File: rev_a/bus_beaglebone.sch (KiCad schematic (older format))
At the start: 39 parts, among them J1 TERMINATE_JUMPER, J2 LED_JUMPER, Q1 FQP47P06, SW1 MJTP1243, U1 74HCT08, U2 MCP2562, U3 ATMEGA324_DIP40, X1 16MHz, X2 OSHW_LOGO

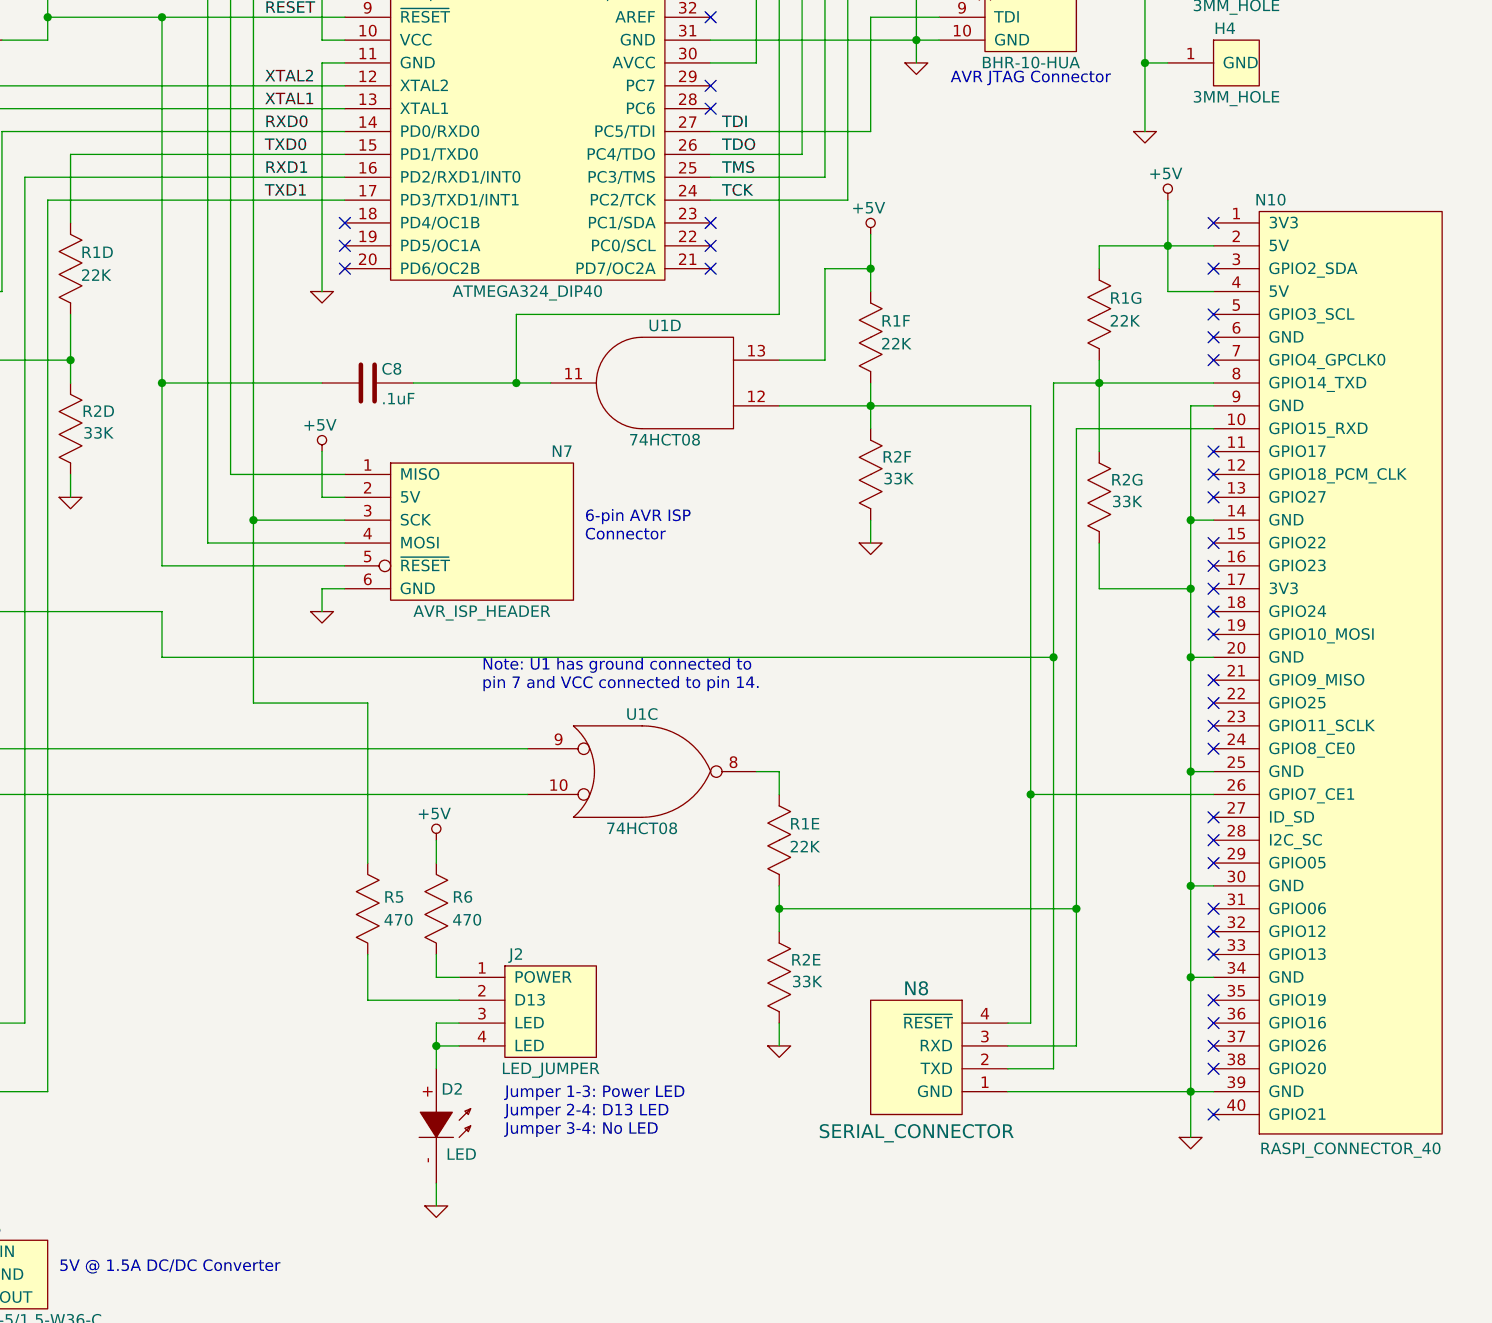
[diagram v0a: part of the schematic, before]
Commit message: Updated again.
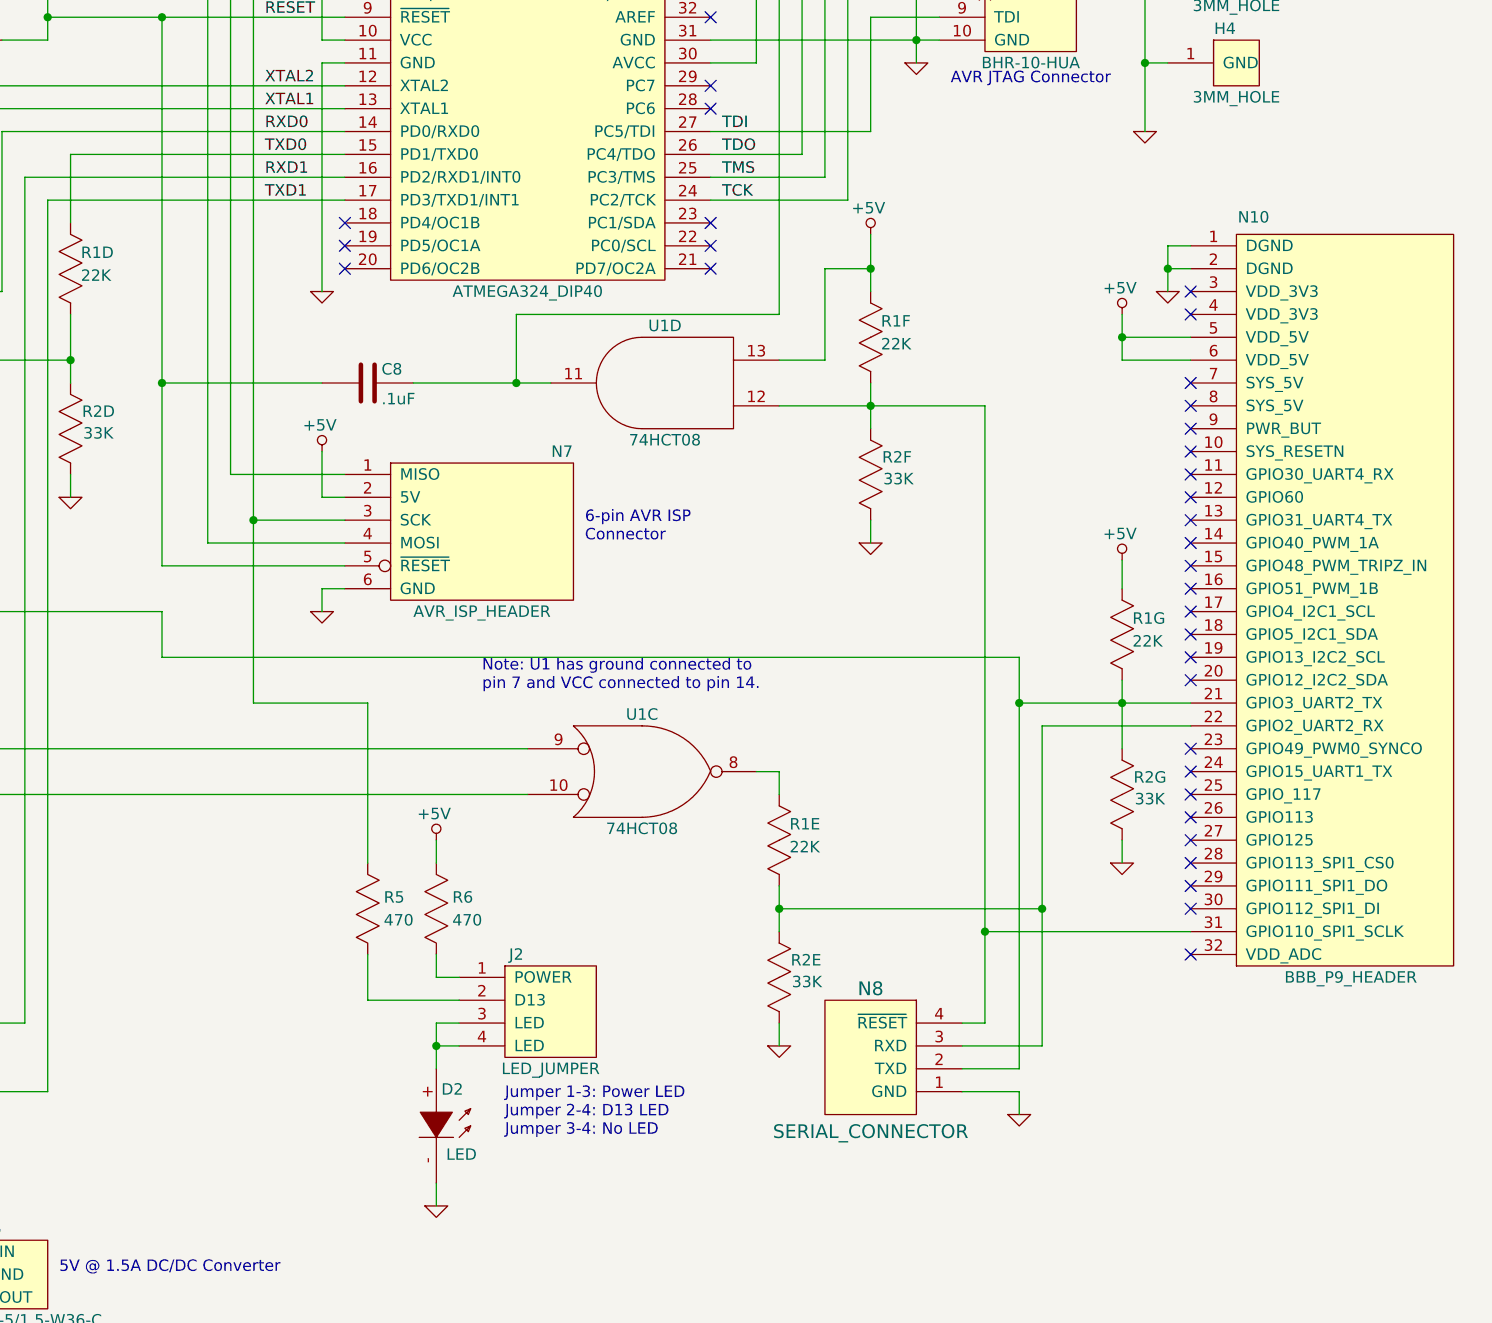
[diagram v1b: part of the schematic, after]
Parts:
- removed N10: RASPI_CONNECTOR_40, symbol RASPI_CONNECTOR_40
- added N10: BBB_P9_HEADER, symbol BBB_P9_HEADER
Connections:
- net +5V: now also N10.5 (VDD_5V), N10.6 (VDD_5V)
- net GND: now also N10.1 (DGND), N10.2 (DGND)
- net at N5.5 (RXD), N8.2 (TXD), R1.8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: now also N10.21 (GPIO3_UART2_TX)
- net at N8.3 (RXD), R1.6, R2.6: now also N10.22 (GPIO2_UART2_RX)
- net at N8.4 (~RESET), R1.7, R2.7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: now also N10.31 (GPIO110_SPI1_SCLK)
- no-connect marks 63 -> 60
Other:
- moved on the sheet: N8, R1G, R2G
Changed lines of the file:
@@
 L GND #PWR09
 U 1 1 53E41588
-P 9300 6600
-F 0 "#PWR09" H 9300 6600 30  0001 C CNN
-F 1 "GND" H 9300 6530 30  0001 C CNN
-F 2 "" H 9300 6600 60  0000 C CNN
-F 3 "" H 9300 6600 60  0000 C CNN
-	1    9300 6600
+P 8550 6500
+F 0 "#PWR09" H 8550 6500 30  0001 C CNN
+F 1 "GND" H 8550 6430 30  0001 C CNN
+F 2 "" H 8550 6500 60  0000 C CNN
+F 3 "" H 8550 6500 60  0000 C CNN
+	1    8550 6500
 	1    0    0    -1
 $EndComp
@@
 L +5V #PWR017
 U 1 1 53E51681
-P 9200 2500
-F 0 "#PWR017" H 9200 2590 20  0001 C CNN
-F 1 "+5V" H 9190 2615 50  0000 C CNN
-F 2 "" H 9200 2500 60  0000 C CNN
-F 3 "" H 9200 2500 60  0000 C CNN
-	1    9200 2500
+P 9000 3000
+F 0 "#PWR017" H 9000 3090 20  0001 C CNN
+F 1 "+5V" H 8990 3115 50  0000 C CNN
+F 2 "" H 9000 3000 60  0000 C CNN
+F 3 "" H 9000 3000 60  0000 C CNN
+	1    9000 3000
 	1    0    0    -1
 $EndComp
@@
 	1    0    0    -1
 $EndComp
-$Comp
-L RASPI_CONNECTOR_40 N10
-U 1 1 53E65B95
-P 10000 4450
-F 0 "N10" H 9650 6400 50  0000 C CNN
-F 1 "RASPI_CONNECTOR_40" H 10000 2250 50  0000 C CNN
-F 2 "" H 10000 5050 60  0000 C CNN
-F 3 "" H 10000 5050 60  0000 C CNN
-	1    10000 4450
-	1    0    0    -1
-$EndComp
-NoConn ~ 9400 2600
-NoConn ~ 9400 2800
-NoConn ~ 9400 3000
-NoConn ~ 9400 3100
-NoConn ~ 9400 3200
-NoConn ~ 9400 3600
-NoConn ~ 9400 3700
-NoConn ~ 9400 3800
-NoConn ~ 9400 4000
-NoConn ~ 9400 4100
-NoConn ~ 9400 4200
-NoConn ~ 9400 4300
-NoConn ~ 9400 4400
-NoConn ~ 9400 4600
-NoConn ~ 9400 4700
-NoConn ~ 9400 4800
-NoConn ~ 9400 4900
-NoConn ~ 9400 5200
-NoConn ~ 9400 5300
-NoConn ~ 9400 5400
-NoConn ~ 9400 5600
-NoConn ~ 9400 5700
-NoConn ~ 9400 5800
-NoConn ~ 9400 6000
-NoConn ~ 9400 6100
-NoConn ~ 9400 6200
-NoConn ~ 9400 6300
-NoConn ~ 9400 6500
 Text Notes 6650 4000 0    50   ~ 0
 6-pin AVR ISP\nConnector
@@
 L SERIAL_CONNECTOR N8
 U 1 1 53E7BE34
-P 8100 6250
-F 0 "N8" H 8100 6550 60  0000 C CNN
-F 1 "SERIAL_CONNECTOR" H 8100 5925 60  0000 C CNN
-F 2 "" H 8100 6250 60  0000 C CNN
-F 3 "" H 8100 6250 60  0000 C CNN
-	1    8100 6250
+P 7900 6250
+F 0 "N8" H 7900 6550 60  0000 C CNN
+F 1 "SERIAL_CONNECTOR" H 7900 5925 60  0000 C CNN
+F 2 "" H 7900 6250 60  0000 C CNN
+F 3 "" H 7900 6250 60  0000 C CNN
+	1    7900 6250
 	-1   0    0    -1
 $EndComp
@@
 	1300 3100 1900 3100
 Wire Wire Line
-	9300 3400 9300 6600
-Wire Wire Line
-	9300 3400 9400 3400
-Wire Wire Line
-	9400 5000 9300 5000
-Connection ~ 9300 5000
-Connection ~ 9300 5500
-Wire Wire Line
-	9400 3900 9300 3900
-Connection ~ 9300 3900
-Wire Wire Line
-	8800 3500 9400 3500
+	8650 4800 9300 4800
 Wire Wire Line
 	7500 5500 7500 5700
@@
 	3500 6900 3500 7300
 Wire Wire Line
-	9200 2900 9400 2900
-Wire Wire Line
-	9200 2500 9200 2900
-Wire Wire Line
-	8900 2700 9400 2700
-Connection ~ 9200 2700
+	9000 3200 9300 3200
+Wire Wire Line
+	9000 3000 9000 3200
 Wire Wire Line
 	2300 6400 2200 6400
@@
 	1600 5500 1600 5700
 Wire Wire Line
-	8700 3300 9400 3300
+	8550 4700 9300 4700
 Wire Wire Line
 	3500 1500 4300 1500
@@
 	1300 3200 4400 3200
 Wire Wire Line
-	8800 3500 8800 6200
-Wire Wire Line
-	8800 5600 7500 5600
+	8650 4800 8650 6200
+Wire Wire Line
+	8650 5600 7500 5600
 Connection ~ 7500 5600
 Wire Wire Line
@@
 	5200 1600 5600 1600
 Wire Wire Line
-	9400 5100 8600 5100
-Wire Wire Line
-	8600 3400 8600 6100
+	9300 5700 8400 5700
+Wire Wire Line
+	8400 3400 8400 6100
 Wire Wire Line
 	7500 1400 8200 1400
@@
 	6350 3000 7500 3000
 Wire Wire Line
-	7500 3400 8600 3400
+	7500 3400 8400 3400
 Wire Wire Line
 	5200 1600 5200 4700
@@
 	7900 3300 7900 3500
 Connection ~ 7900 3400
-Wire Wire Line
-	8900 2700 8900 2800
-Wire Wire Line
-	9400 4500 9300 4500
-Connection ~ 9300 4500
 Wire Wire Line
 	7500 3000 7500 1400
@@
 	7700 2400 7200 2400
 Wire Wire Line
-	8900 4200 9300 4200
-Connection ~ 9300 4200
-Wire Wire Line
-	8900 4200 8900 4000
-Wire Wire Line
-	8500 6400 9400 6400
-Connection ~ 9300 6400
-Wire Wire Line
-	9400 5500 9300 5500
-Wire Wire Line
-	9400 5900 9300 5900
-Connection ~ 9300 5900
-Wire Wire Line
-	4800 4500 8700 4500
-Wire Wire Line
-	8700 3300 8700 6300
-Wire Wire Line
-	8900 3200 8900 3600
-Connection ~ 8900 3300
+	9000 5400 9000 5300
+Wire Wire Line
+	4800 4500 8550 4500
+Wire Wire Line
+	8550 4500 8550 6300
+Wire Wire Line
+	9000 4600 9000 4900
+Connection ~ 9000 4700
 Wire Wire Line
 	4800 4100 5600 4100
@@
 	5500 3300 4800 3300
 Wire Wire Line
-	8600 6100 8500 6100
-Connection ~ 8600 5100
-Wire Wire Line
-	8700 6300 8500 6300
-Connection ~ 8700 4500
-Wire Wire Line
-	8800 6200 8500 6200
-Connection ~ 8800 5600
+	8400 6100 8300 6100
+Connection ~ 8400 5700
+Wire Wire Line
+	8550 6300 8300 6300
+Wire Wire Line
+	8650 6200 8300 6200
+Connection ~ 8650 5600
 Text Label 1150 7100 0    50   ~ 0
 BAT+
@@
 L R_VERT_SIP8 R1
 U 7 1 53E80F50
-P 8900 3000
-F 0 "R1" H 8945 3070 50  0000 L CNN
-F 1 "22K" H 8945 2970 50  0000 L CNN
-F 2 "" H 8900 3000 50  0000 C CNN
-F 3 "" H 8900 3000 50  0000 C CNN
-	7    8900 3000
+P 9000 4400
+F 0 "R1" H 9045 4470 50  0000 L CNN
+F 1 "22K" H 9045 4370 50  0000 L CNN
+F 2 "" H 9000 4400 50  0000 C CNN
+F 3 "" H 9000 4400 50  0000 C CNN
+	7    9000 4400
 	1    0    0    -1
 $EndComp
@@
 L R_VERT_SIP8 R2
 U 7 1 53E81C9B
-P 8900 3800
-F 0 "R2" H 8850 3725 50  0000 R CNN
-F 1 "33K" H 8845 3820 50  0000 R CNN
-F 2 "" H 8900 3800 50  0000 C CNN
-F 3 "" H 8900 3800 50  0000 C CNN
-	7    8900 3800
+P 9000 5100
+F 0 "R2" H 8950 5025 50  0000 R CNN
+F 1 "33K" H 8945 5120 50  0000 R CNN
+F 2 "" H 9000 5100 50  0000 C CNN
+F 3 "" H 9000 5100 50  0000 C CNN
+	7    9000 5100
 	-1   0    0    1
 $EndComp
@@
 	-1   0    0    1
 $EndComp
+$Comp
+L BBB_P9_HEADER N10
+U 1 1 53E8703D
+P 10000 4250
+F 0 "N10" H 9575 5925 50  0000 C CNN
+F 1 "BBB_P9_HEADER" H 10000 2600 50  0000 C CNN
+F 2 "" H 10000 4550 60  0000 C CNN
+F 3 "" H 10000 4550 60  0000 C CNN
+	1    10000 4250
+	1    0    0    -1
+$EndComp
+Wire Wire Line
+	9300 3100 9000 3100
+Connection ~ 9000 3100
+Wire Wire Line
+	9300 2700 9200 2700
+Wire Wire Line
+	9200 2700 9200 2900
+Wire Wire Line
+	9200 2800 9300 2800
+$Comp
+L GND #PWR031
+U 1 1 53E8748B
+P 9200 2900
+F 0 "#PWR031" H 9200 2900 30  0001 C CNN
+F 1 "GND" H 9200 2830 30  0001 C CNN
+F 2 "" H 9200 2900 60  0000 C CNN
+F 3 "" H 9200 2900 60  0000 C CNN
+	1    9200 2900
+	1    0    0    -1
+$EndComp
+Connection ~ 9200 2800
+Connection ~ 8550 4700
+$Comp
+L GND #PWR032
+U 1 1 53E87E15
+P 9000 5400
+F 0 "#PWR032" H 9000 5400 30  0001 C CNN
+F 1 "GND" H 9000 5330 30  0001 C CNN
+F 2 "" H 9000 5400 60  0000 C CNN
+F 3 "" H 9000 5400 60  0000 C CNN
+	1    9000 5400
+	1    0    0    -1
+$EndComp
+$Comp
+L +5V #PWR033
+U 1 1 53E87FB6
+P 9000 4075
+F 0 "#PWR033" H 9000 4165 20  0001 C CNN
+F 1 "+5V" H 8990 4190 50  0000 C CNN
+F 2 "" H 9000 4075 60  0000 C CNN
+F 3 "" H 9000 4075 60  0000 C CNN
+	1    9000 4075
+	1    0    0    -1
+$EndComp
+Wire Wire Line
+	9000 4200 9000 4075
+NoConn ~ 9300 2900
+NoConn ~ 9300 3000
+NoConn ~ 9300 3300
+NoConn ~ 9300 3400
+NoConn ~ 9300 3500
+NoConn ~ 9300 3600
+NoConn ~ 9300 3700
+NoConn ~ 9300 3800
+NoConn ~ 9300 3900
+NoConn ~ 9300 4000
+NoConn ~ 9300 4100
+NoConn ~ 9300 4200
+NoConn ~ 9300 4300
+NoConn ~ 9300 4400
+NoConn ~ 9300 4500
+NoConn ~ 9300 4600
+NoConn ~ 9300 4900
+NoConn ~ 9300 5000
+NoConn ~ 9300 5800
+NoConn ~ 9300 5600
+NoConn ~ 9300 5500
+NoConn ~ 9300 5400
+NoConn ~ 9300 5300
+NoConn ~ 9300 5200
+NoConn ~ 9300 5100
+Wire Wire Line
+	8550 6500 8550 6400
+Wire Wire Line
+	8550 6400 8300 6400
 $EndSCHEMATC
